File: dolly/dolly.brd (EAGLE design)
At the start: 135.9 x 158.8 mm, 31 parts, among them U1 ATTINY85-20P

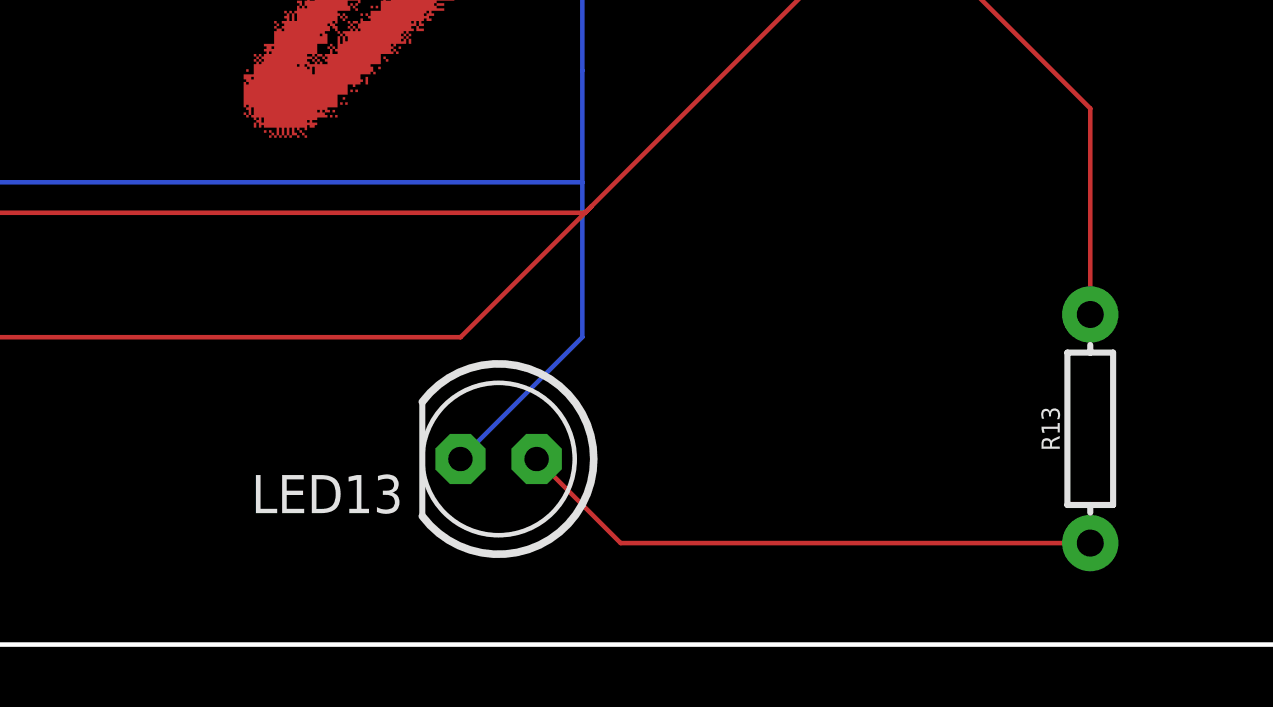
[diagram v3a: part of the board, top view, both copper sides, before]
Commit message: DOLLY BADGE OK LOL
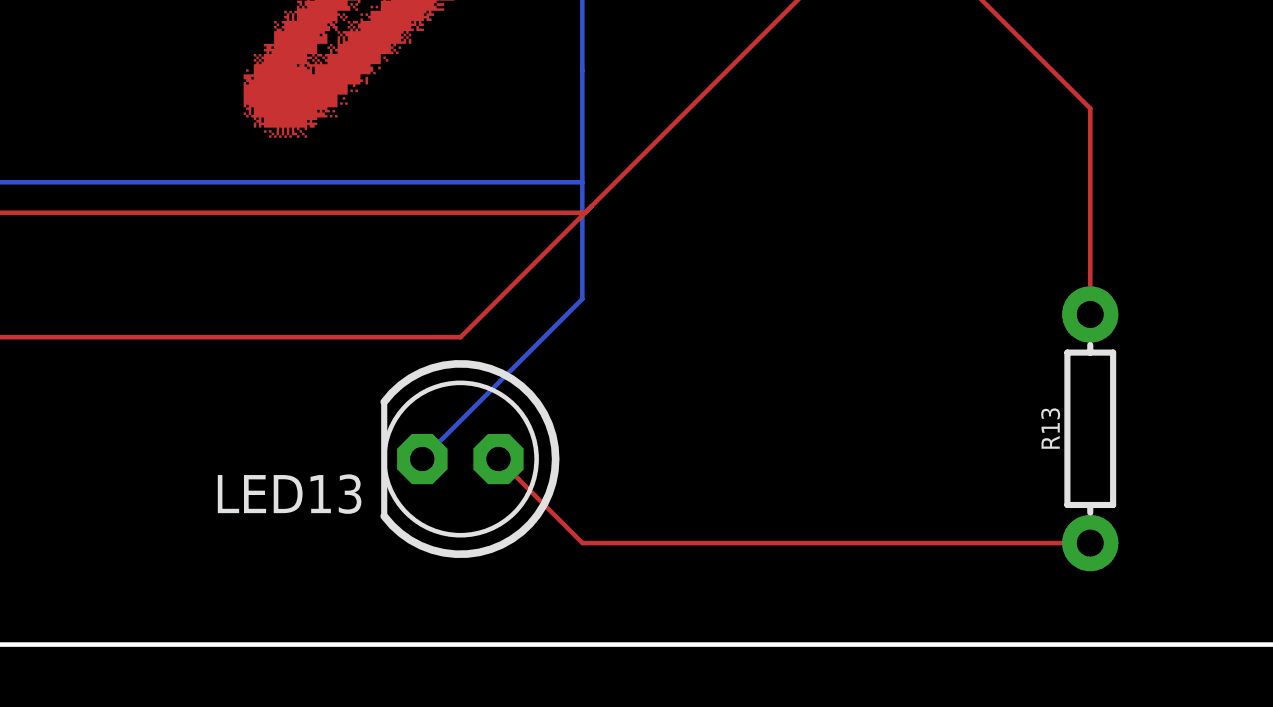
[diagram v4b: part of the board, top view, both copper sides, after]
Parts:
- moved LED13 1.27 mm to (68.2, -6.52)
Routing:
- net N$16: track 19.6 -> 20.9 mm
- net N$4: track 987.9 -> 988.4 mm
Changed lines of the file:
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@@
 <element name="LED11" library="adafruit" package="LED5MM" value="" x="108.781978125" y="66.206140625" rot="R270"/>
 <element name="LED12" library="adafruit" package="LED5MM" value="" x="108.951421875" y="33.865825" rot="R270"/>
-<element name="LED13" library="adafruit" package="LED5MM" value="" x="69.49918125" y="-6.516009375" rot="R180"/>
+<element name="LED13" library="adafruit" package="LED5MM" value="" x="68.22918125" y="-6.516009375" rot="R180"/>
 <element name="LED14" library="adafruit" package="LED5MM" value="" x="-7.113321875" y="-3.975503125" rot="R180"/>
 <element name="LED2" library="adafruit" package="LED5MM" value="" x="24.633371875" y="-6.091196875" rot="R180"/>
@@
 <wire x1="72.293159375" y1="6.434021875" x2="72.293159375" y2="30.39229375" width="0.1524" layer="16"/>
 <wire x1="71.874809375" y1="30.39229375" x2="71.95946875" y2="30.39229375" width="0.1524" layer="16"/>
-<wire x1="68.22918125" y1="-6.516009375" x2="72.293159375" y2="-2.45203125" width="0.1524" layer="16"/>
+<wire x1="66.95918125" y1="-6.516009375" x2="72.293159375" y2="-1.18203125" width="0.1524" layer="16"/>
 <wire x1="71.874809375" y1="30.39229375" x2="77.46225" y2="30.39229375" width="0.1524" layer="16"/>
 <wire x1="23.363371875" y1="-6.091196875" x2="32.16363125" y2="2.7090625" width="0.1524" layer="16"/>
 <wire x1="32.16363125" y1="2.7090625" x2="32.33943125" y2="2.7090625" width="0.1524" layer="16"/>
 <wire x1="32.33943125" y1="2.7090625" x2="72.293159375" y2="2.7090625" width="0.1524" layer="16"/>
-<wire x1="72.293159375" y1="-2.45203125" x2="72.293159375" y2="2.7090625" width="0.1524" layer="16"/>
+<wire x1="72.293159375" y1="-1.18203125" x2="72.293159375" y2="2.7090625" width="0.1524" layer="16"/>
 <wire x1="-8.383321875" y1="-3.975503125" x2="-1.69875625" y2="2.7090625" width="0.1524" layer="16"/>
 <wire x1="-1.69875625" y1="2.7090625" x2="32.33943125" y2="2.7090625" width="0.1524" layer="16"/>
@@
 <contactref element="R13" pad="P$1"/>
 <contactref element="LED13" pad="A"/>
-<wire x1="89.22415625" y1="-9.317609375" x2="73.57078125" y2="-9.317609375" width="0.1524" layer="1"/>
-<wire x1="73.57078125" y1="-9.317609375" x2="70.76918125" y2="-6.516009375" width="0.1524" layer="1"/>
+<wire x1="89.22415625" y1="-9.317609375" x2="72.30078125" y2="-9.317609375" width="0.1524" layer="1"/>
+<wire x1="72.30078125" y1="-9.317609375" x2="69.49918125" y2="-6.516009375" width="0.1524" layer="1"/>
 </signal>
 <signal name="N$17">

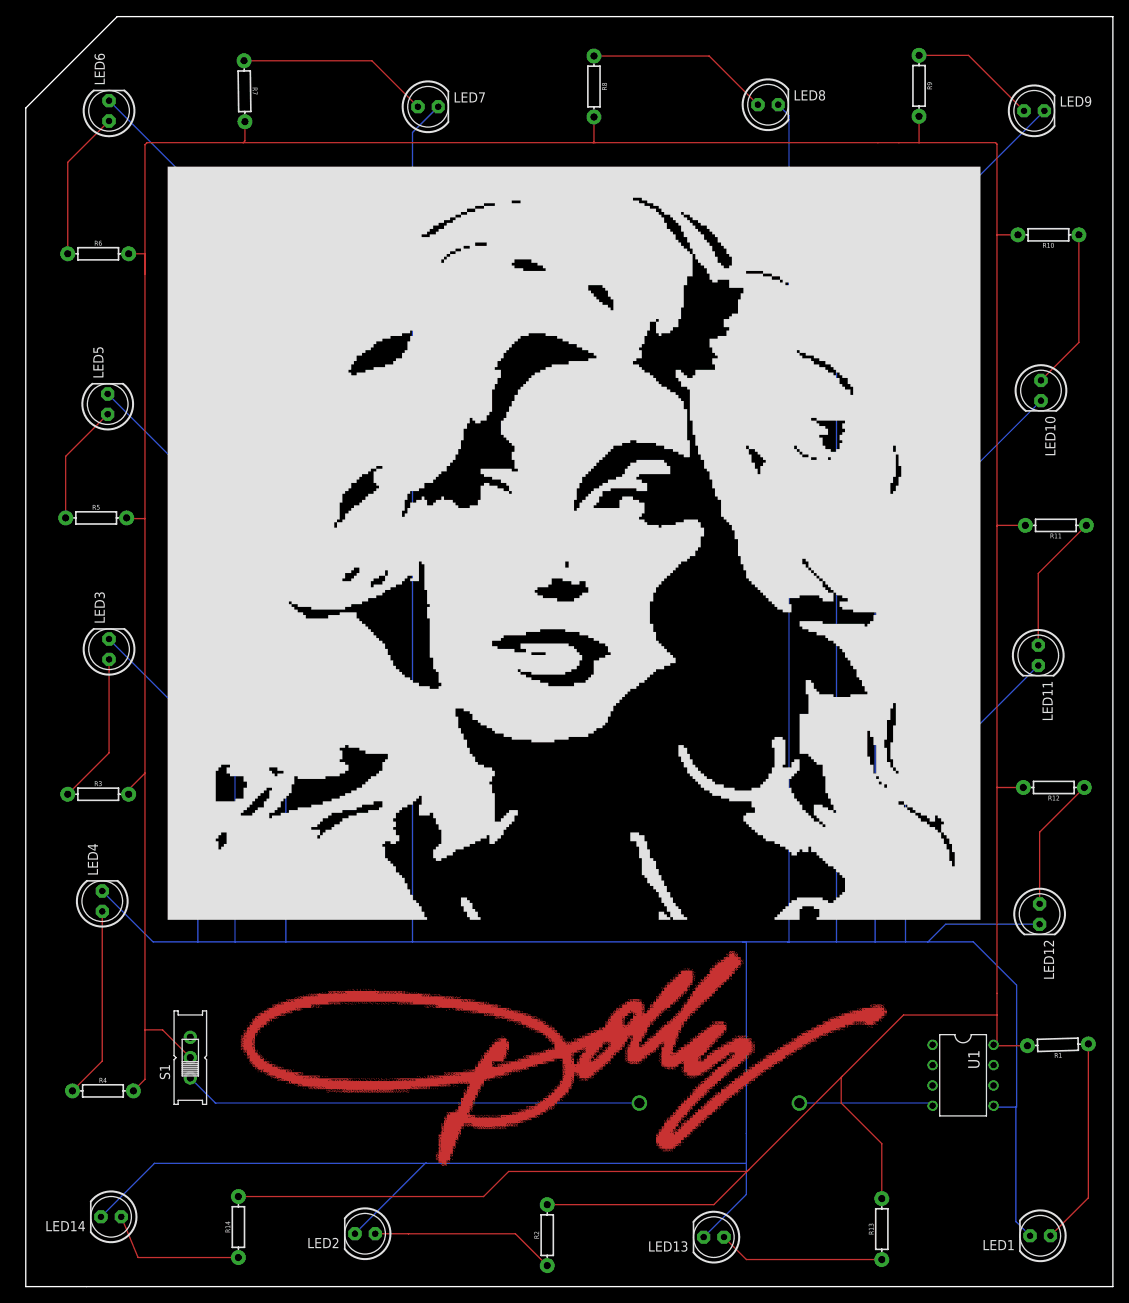
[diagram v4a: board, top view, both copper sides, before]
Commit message: DOLLY BADGE OK LOL
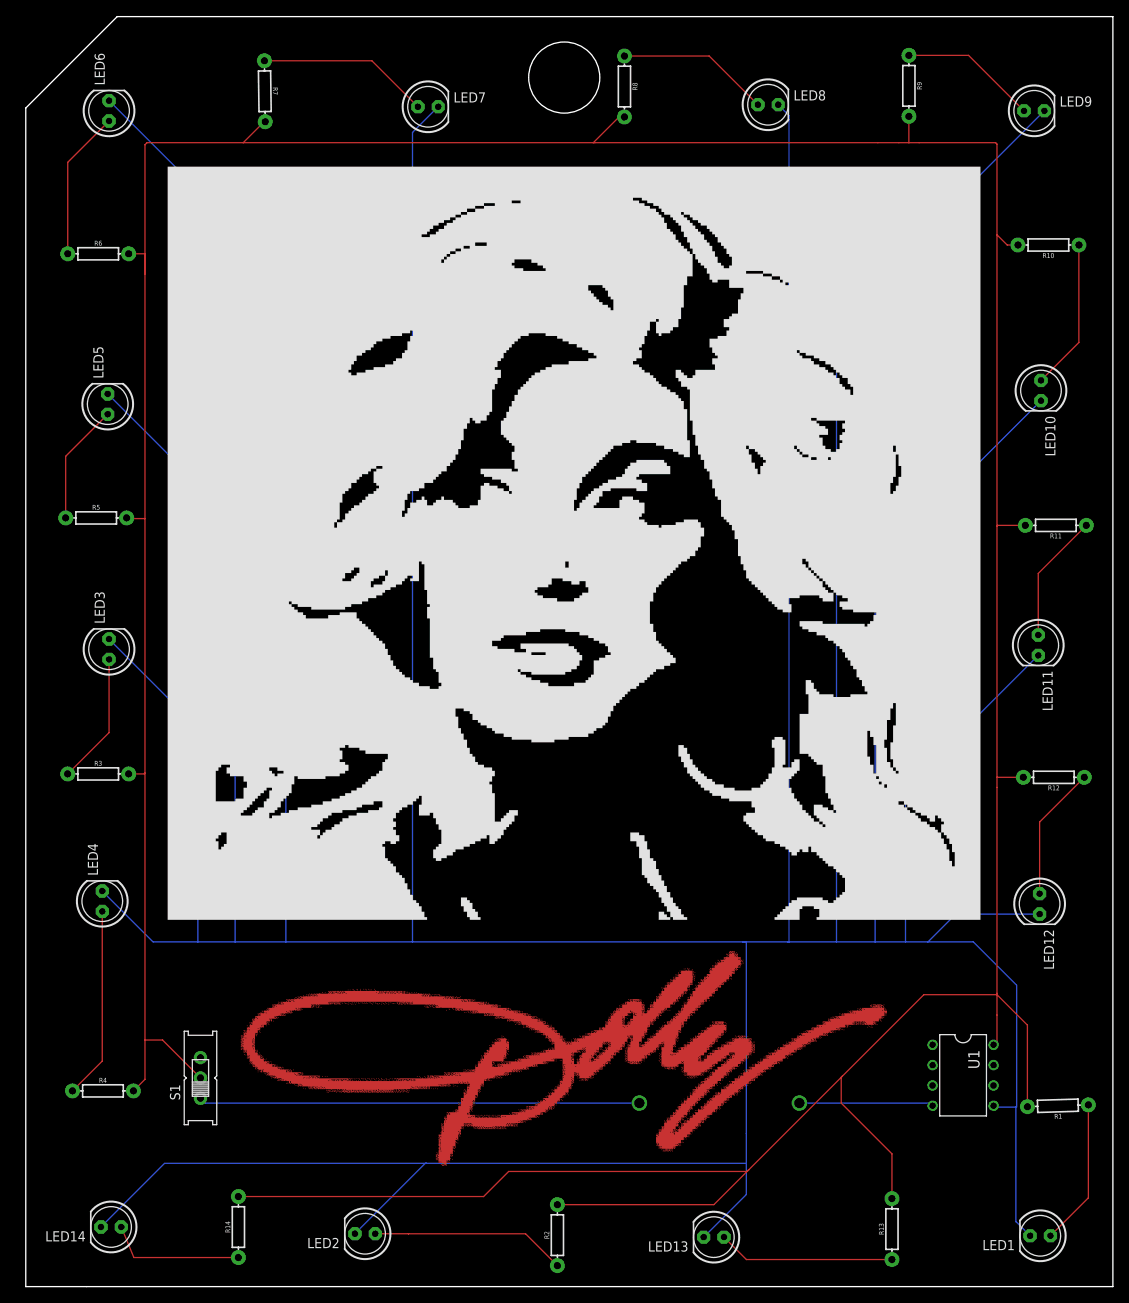
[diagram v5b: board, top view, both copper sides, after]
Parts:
- moved R1 7.62 mm to (111.2, 9.90)
- moved R8 3.81 mm to (57.1, 137.3)
- moved S1 2.84 mm to (4.06, 13.4)
- moved R7 2.54 mm to (12.1, 136.7)
- moved R3 2.54 mm to (-8.72, 51.4)
- moved R13 1.27 mm to (90.5, -5.51)
- moved R12 1.27 mm to (110.7, 51.0)
- moved LED14 1.27 mm to (-7.11, -5.25)
- moved LED11 1.27 mm to (108.8, 67.5)
- moved LED12 1.27 mm to (109.0, 35.1)
- moved R10 1.27 mm to (110.1, 117.5)
- moved R2 1.27 mm to (48.7, -6.27)
- moved R9 1.27 mm to (92.6, 137.4)
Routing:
- net N$6: track 527.8 -> 543.6 mm
- net N$1: track 25.9 -> 18.3 mm
- net N$11: track 23.0 -> 19.2 mm
- net N$3: track 19.0 -> 16.5 mm
- net N$10: track 24.1 -> 21.6 mm
- net N$2: track 58.1 -> 55.8 mm
- net N$4: track 988.4 -> 990.7 mm
- net N$16: track 20.9 -> 22.2 mm
- net N$18: track 23.2 -> 24.4 mm
- net N$14: track 17.5 -> 16.2 mm
- net N$13: track 20.2 -> 18.9 mm
- net N$12: track 16.0 -> 17.3 mm
- net N$17: track 18.0 -> 17.2 mm

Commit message: resize dolly badge
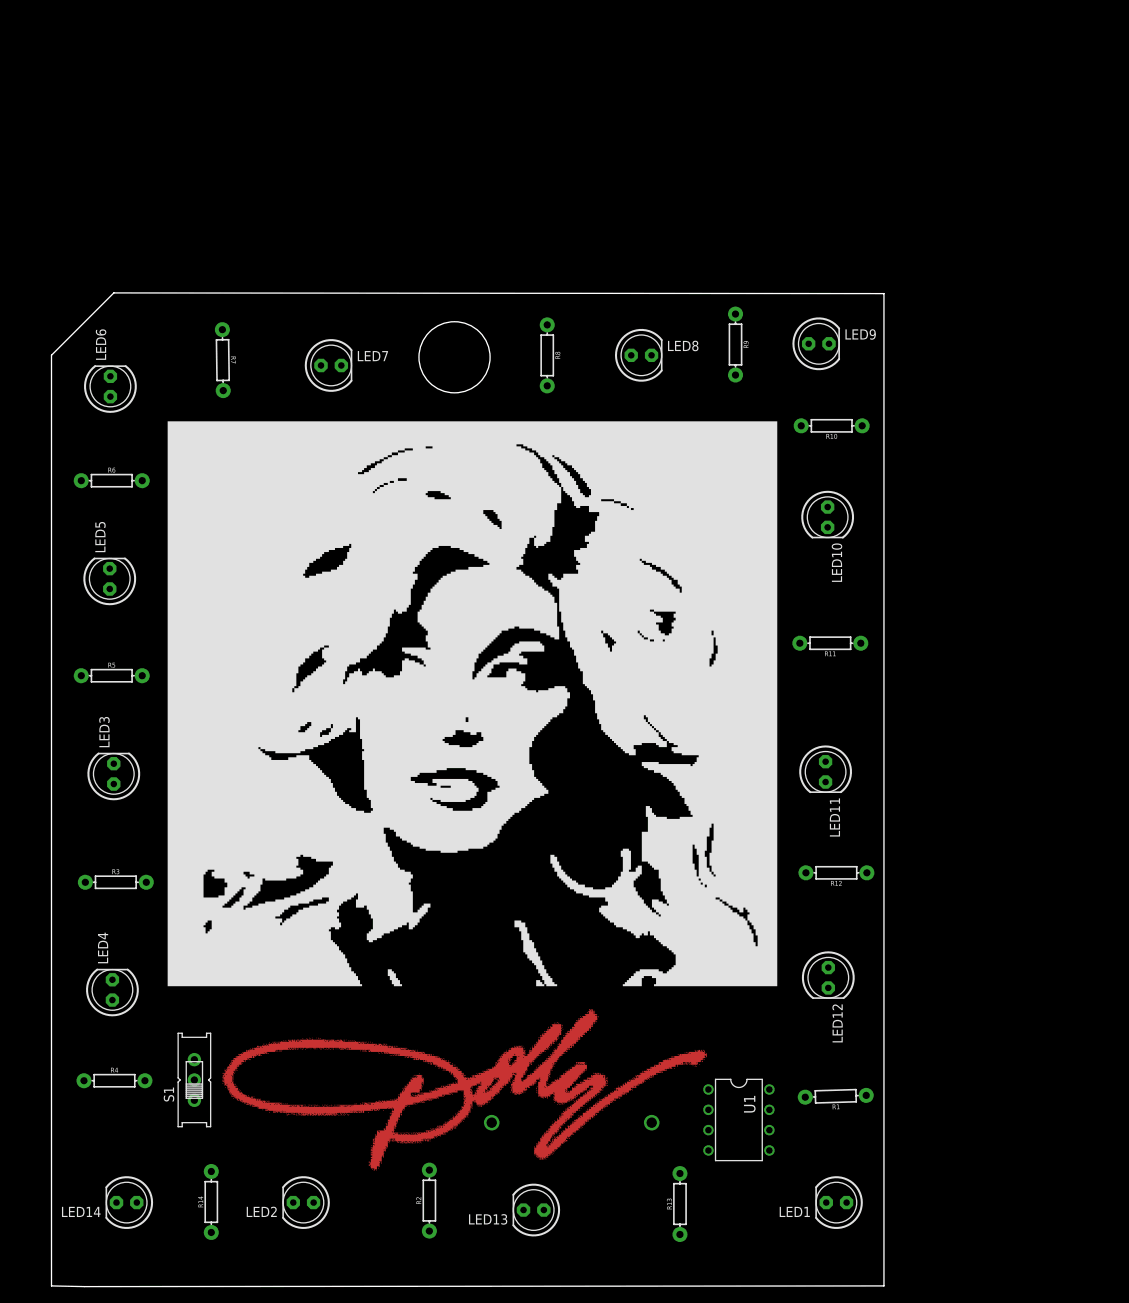
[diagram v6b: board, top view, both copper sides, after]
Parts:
- moved LED9 39.7 mm to (81.4, 105.2)
- moved R9 38.9 mm to (70.9, 105.1)
- moved R10 35.3 mm to (83.0, 94.9)
- moved LED8 35.1 mm to (59.2, 103.7)
- moved R8 35.0 mm to (47.4, 103.7)
- moved LED7 34.5 mm to (20.4, 102.4)
- moved LED6 34.5 mm to (-7.20, 99.8)
- moved R7 34.0 mm to (6.85, 103.1)
- moved R11 31.8 mm to (82.8, 67.7)
- moved LED10 31.0 mm to (82.5, 83.5)
- moved LED11 30.9 mm to (82.2, 51.6)
- moved R12 29.7 mm to (83.6, 39.0)
- moved U1 28.6 mm to (71.4, 8.13)
- moved R6 28.4 mm to (-7.03, 88.0)
- moved LED12 28.0 mm to (82.5, 25.9)
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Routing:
- net N$4: track 990.7 -> 0.00 mm
- net N$6: track 543.6 -> 0.00 mm
- net N$2: track 55.8 -> 0.00 mm
- net N$18: track 24.4 -> 0.01 mm
- net N$7: track 24.0 -> 0.00 mm
- net N$16: track 22.2 -> 0.00 mm
- net N$10: track 21.6 -> 0.00 mm
- net N$11: track 19.2 -> 0.00 mm
- net N$13: track 18.9 -> 0.00 mm
- net N$9: track 18.7 -> 0.00 mm
- net N$1: track 18.3 -> 0.00 mm
- net N$5: track 17.3 -> 0.00 mm
- net N$12: track 17.3 -> 0.00 mm
- net N$17: track 17.2 -> 0.00 mm
- net N$15: track 16.9 -> 0.00 mm
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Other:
- board size 135.9 x 158.8 mm -> 104.1 x 124.2 mm
- board text added: "https://github.com/littlefoot22/badges/tree/master/dolly"

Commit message: resize dolly badge
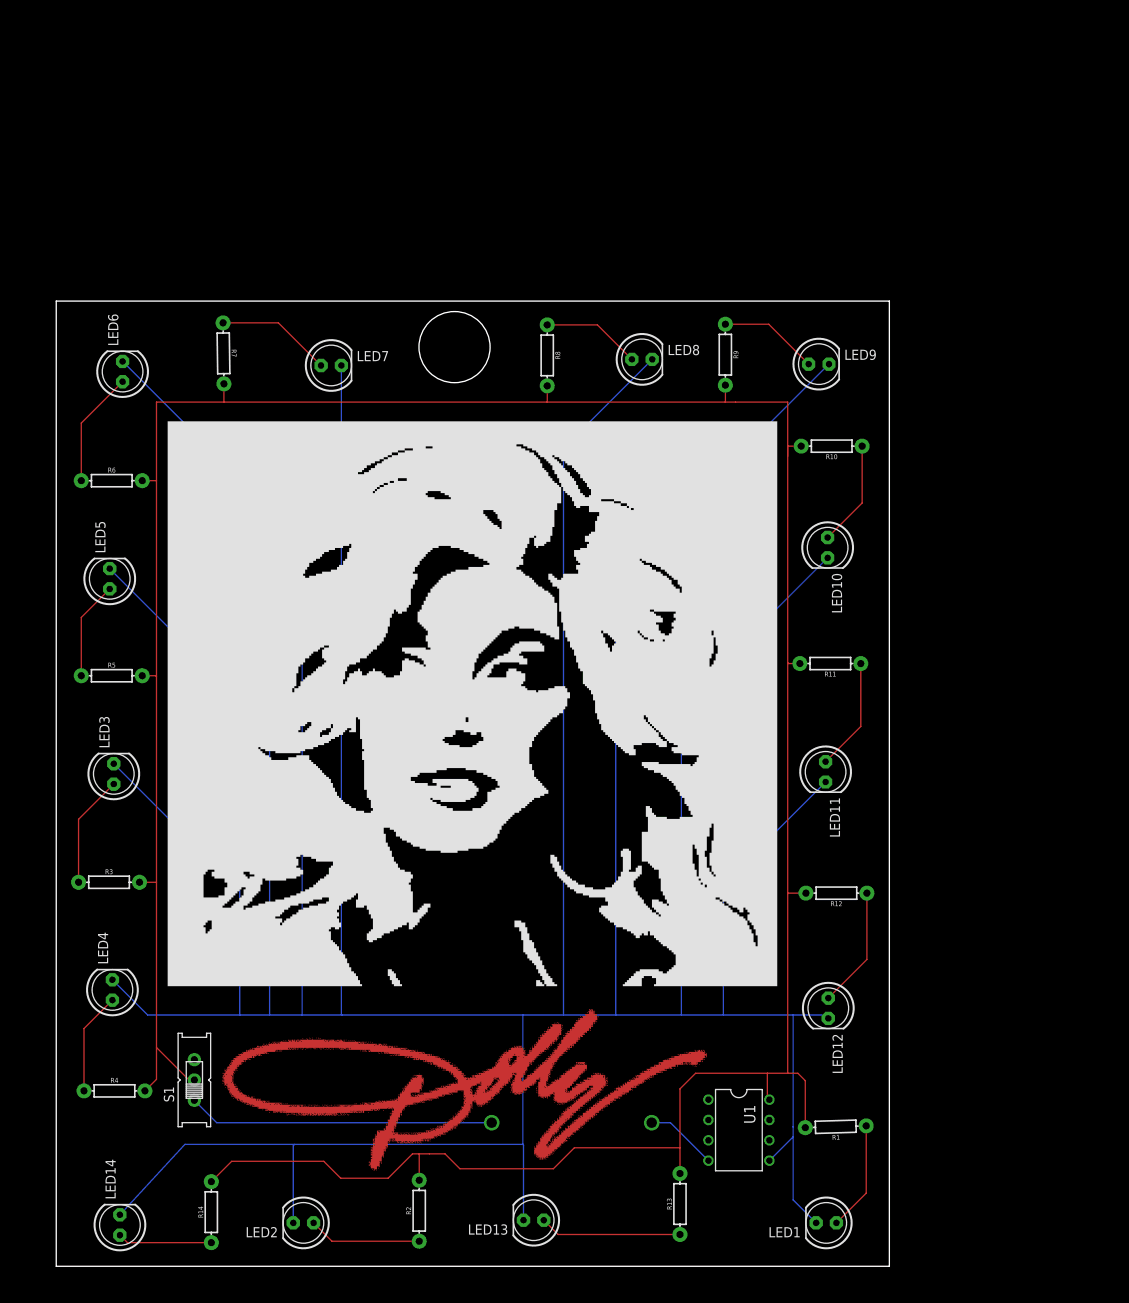
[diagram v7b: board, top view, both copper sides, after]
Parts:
- moved LED10 3.81 mm to (82.5, 79.7)
- moved R1 3.81 mm to (83.5, 7.28)
- moved LED12 3.81 mm to (82.5, 22.1)
- moved LED14 2.92 mm to (-6.01, -4.99), turned to 90 degrees
- moved LED1 2.84 mm to (82.3, -4.74)
- moved R10 2.54 mm to (83.0, 92.4)
- moved R12 2.54 mm to (83.6, 36.5)
- moved LED2 2.54 mm to (16.9, -4.74)
- moved LED9 2.54 mm to (81.4, 102.6)
- moved R11 2.54 mm to (82.8, 65.2)
- moved LED6 2.41 mm to (-5.68, 101.7)
- moved R2 1.80 mm to (31.4, -3.22)
- moved R9 1.80 mm to (69.7, 103.8)
- moved R4 1.27 mm to (-6.69, 11.8)
- moved R14 1.27 mm to (5.41, -3.39)
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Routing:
- net N$4: track 0.00 -> 765.0 mm
- net N$6: track 0.00 -> 378.6 mm
- net N$2: track 0.00 -> 38.3 mm
- net N$16: track 0.00 -> 17.8 mm
- net N$15: track 0.00 -> 15.1 mm
- net N$9: track 0.00 -> 14.5 mm
- net N$10: track 0.00 -> 14.5 mm
- net N$18: track 0.01 -> 14.2 mm
- net N$3: track 0.00 -> 14.1 mm
- net N$14: track 0.00 -> 14.1 mm
- net N$1: track 0.00 -> 13.7 mm
- net N$13: track 0.00 -> 13.2 mm
- net N$7: track 0.00 -> 12.8 mm
- net N$12: track 0.00 -> 12.5 mm
- net N$11: track 0.00 -> 12.4 mm
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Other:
- board size 104.1 x 124.2 mm -> 104.1 x 120.6 mm
